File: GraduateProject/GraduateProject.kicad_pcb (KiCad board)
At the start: 2 copper layers, 90 x 80 mm, 143 parts, among them IC1 PIC16C620A-04/SS, IC2 PIC16C620A-04/SS, J1 Conn_01x05_Pin, J2 Conn_01x04_Pin, J5 Conn_01x04_Pin, J6 Conn_01x04_Pin, J7 Conn_01x05_Pin, J8 Conn_01x05_Pin, Q1 MMBT2222A, Q10 IMX1T110, Q11 MMBT2222A, Q12 IMX1T110, Q13 IMX1T110, Q14 IMX1T110, Q15 IMX1T110, Q16 MMBT2222A, Q17 MMBT2222A, Q18 MMBT2222A, Q19 MMBT2222A, Q2 MMBT2222A, Q20 MMBT2222A, Q21 MMBT2222A, Q22 MMBT2222A, Q23 MMBT3906, Q24 MMBT2222A, Q25 MMBT2222A, Q26 MMBT3906, Q27 MMBT2222A, Q28 MMBT2222A, Q29 MMBT2222A, Q3 MBT3946DW1T1, Q30 MMBT2222A, Q31 MMBT2222A, Q32 MMBT2222A, Q33 MMBT2222A, Q34 MMBT2222A, Q35 MMBT2222A, Q36 MMBT2222A, Q4 MMBT2222A, Q6 IMX1T110, Q7 IMX1T110, Q8 MBT3946DW1T1, Q9 IMX1T110, SW1 SS12D10G3, U2 L7815, U3 L7805, U4 L7805, U5 B0505S-1W, U6 EL357N(D)(TA)-G_C42385002, U7 B0505S-1W

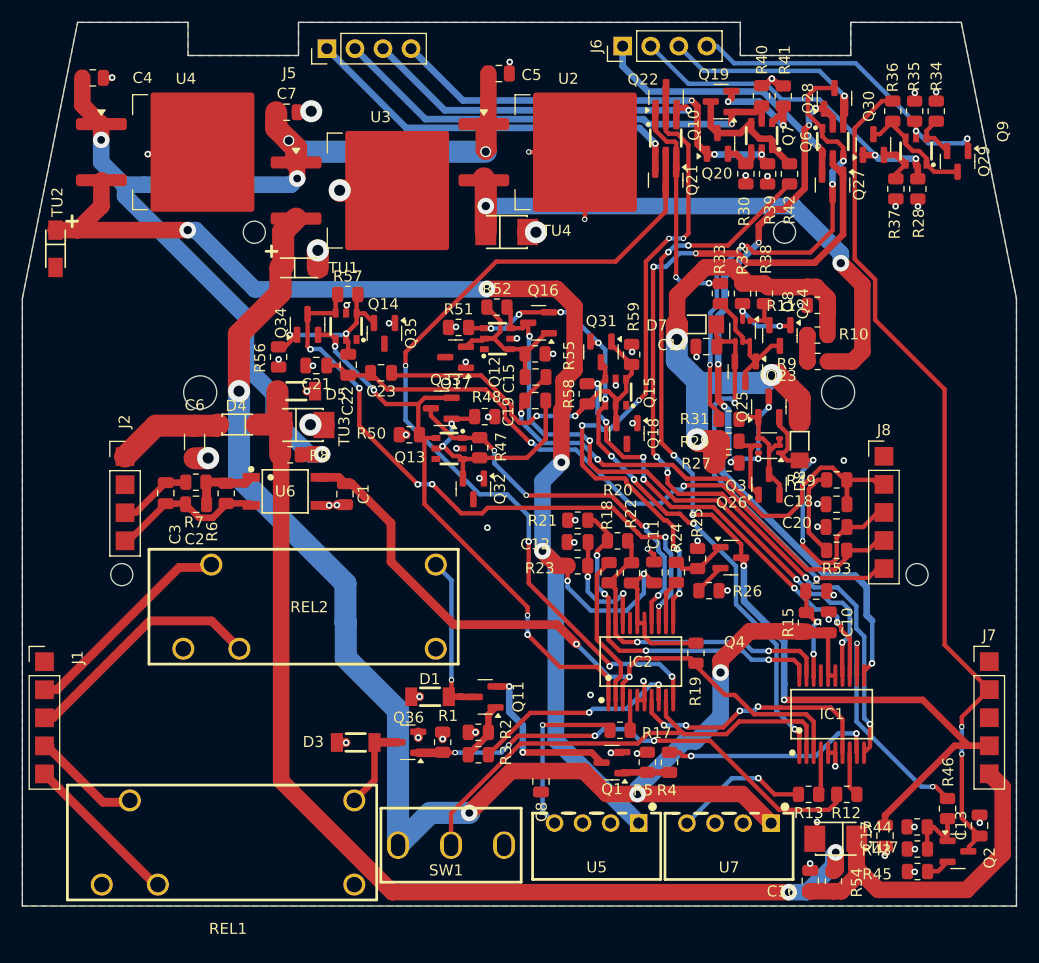
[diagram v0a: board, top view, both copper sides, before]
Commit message: Add files via upload
5/10/25
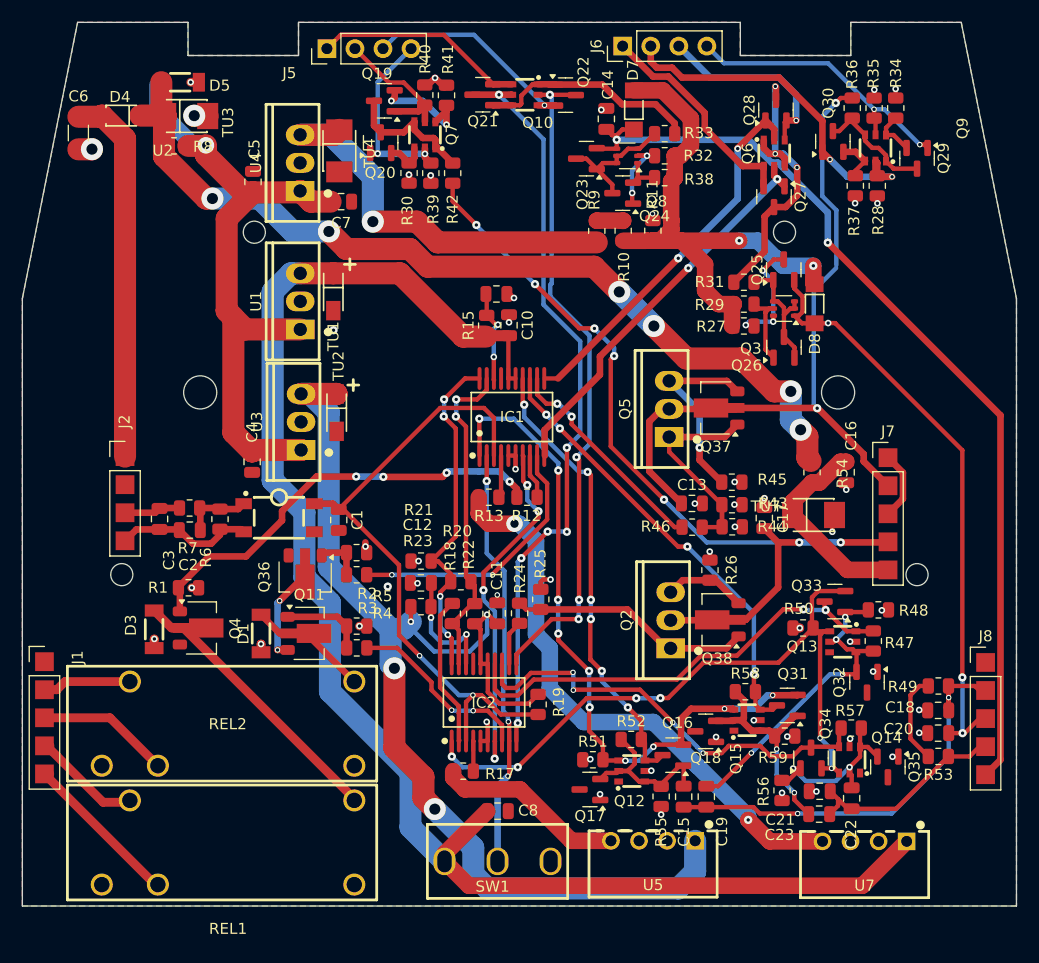
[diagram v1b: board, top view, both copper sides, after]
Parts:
- removed Q1: MMBT2222A, Package_TO_SOT_SMD:SOT-23
- removed U6: EL357N(D)(TA)-G_C42385002, easyeda2kicad:SOP-4_L3.9-W4.4-P2.54-LS7.0-TL
- added Q37: BCX56, Package_TO_SOT_SMD:SOT-89-3, F.Cu at (167.8, 114.9)
- added Q38: BCX56, Package_TO_SOT_SMD:SOT-89-3, F.Cu at (167.9, 134.1)
- added Q5: TIP110G, easyeda2kicad:TO-220-3_L10.0-W4.5-P2.54-L, F.Cu at (163.6, 115.0)
- added U1: LM7805T, easyeda2kicad:TO-220-3_L10.0-W4.5-P2.54-L, F.Cu at (130.2, 105.3)
- Q11, Q36, Q4: value MMBT2222A -> BCX56; footprint Package_TO_SOT_SMD:SOT-23 -> Package_TO_SOT_SMD:SOT-89-3
- Q2: value MMBT2222A -> TIP110G; footprint Package_TO_SOT_SMD:SOT-23 -> easyeda2kicad:TO-220-3_L10.0-W4.5-P2.54-L
- U2: value L7815 -> TLP181GB-S; footprint Package_TO_SOT_SMD:TO-263-2 -> easyeda2kicad:SOP-4_L3.7-W4.6-P2.54-LS7.0-TL
- U3: value L7805 -> LM7805T; footprint Package_TO_SOT_SMD:TO-263-2 -> easyeda2kicad:TO-220-3_L10.0-W4.5-P2.54-L
- U4: value L7805 -> L7815CV; footprint Package_TO_SOT_SMD:TO-263-2 -> easyeda2kicad:TO-220-3_L10.0-W4.5-P2.54-L
- moved C22 60.1 mm to (180.1, 150.2)
- moved Q34 60.1 mm to (176.4, 146.6)
- moved R56 60.1 mm to (173.8, 149.5)
- moved Q14 60.1 mm to (179.9, 146.8)
- moved R57 60.1 mm to (180.0, 143.9)
- moved Q35 60.1 mm to (183.4, 147.4)
- moved C21 59.7 mm to (177.2, 149.6)
- moved C23 56.3 mm to (177.1, 151.7), turned to 0 degrees
- moved Q4 48.3 mm to (121.2, 134.8)
- moved U2 42.2 mm to (128.2, 124.8)
- moved R55 41.7 mm to (162.8, 150.1), turned to -90 degrees
- moved Q16 41.0 mm to (163.9, 146.3)
- moved R52 41.0 mm to (160.1, 144.9)
- moved Q12 41.0 mm to (160.2, 147.8)
- moved Q17 41.0 mm to (156.4, 149.4)
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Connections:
- C13 pad 1: Net-(J7-Pin_2) -> /CONNECTORS/BCX56_2
- C2 pad 2: Net-(U6-AN) -> Net-(U2-AN)
- C4 pad 1: Net-(U2-IN) -> Net-(U1-VIN)
- C5 pad 1: Net-(U2-IN) -> Net-(U1-VIN)
- C7 pad 1: Net-(U2-IN) -> Net-(U1-VIN)
- J7 pad 1: unconnected-(J7-Pin_1-Pad1) -> Net-(J7-Pin_1)
- J7 pad 2: Net-(J7-Pin_2) -> /CONNECTORS/BCX56_2
- J7 pad 3: unconnected-(J7-Pin_3-Pad3) -> Net-(J7-Pin_1)
- Q11 pad 2: Net-(Q1-C) -> Net-(D1-C)
- Q11 pad 3: Net-(D1-C) -> Net-(Q11-E)
- Q2 pad 1: Net-(Q2-B) -> /PICs/BCX56_38_1
- Q2 pad 2: Net-(Q2-E) -> /CONNECTORS/CONN_J3_4
- Q2 pad 3: Net-(J7-Pin_2) -> /PICs/BCX56_38_3
- Q36 pad 1: /PICs/RB1_PIC1 -> Net-(Q36-B)
- Q36 pad 2: GND -> Net-(Q11-E)
- Q36 pad 3: Net-(D3-C) -> GND
- Q4 pad 1: Net-(Q4-B) -> /PICs/RB1_PIC1
- Q4 pad 2: Net-(Q4-E) -> Net-(D3-C)
- Q4 pad 3: /CONNECTORS/CONN_J3_4 -> GND
- R24 pad 1: Net-(Q4-B) -> /PICs/BCX56_38_1
- R25 pad 1: Net-(Q4-B) -> /PICs/BCX56_38_1
- R26 pad 1: Net-(Q4-E) -> /PICs/BCX56_38_3
- R36 pad 2: Net-(J7-Pin_2) -> /CONNECTORS/BCX56_2
- R4 pad 2: Net-(Q1-B) -> Net-(Q36-B)
- R43 pad 1: Net-(Q2-B) -> /CONNECTORS/BCX56_1
- R44 pad 1: Net-(Q2-B) -> /CONNECTORS/BCX56_1
- R45 pad 1: Net-(Q2-E) -> /CONNECTORS/BCX56_3
- R46 pad 1: Net-(Q2-B) -> /CONNECTORS/BCX56_1
- R5 pad 2: Net-(Q1-B) -> Net-(Q36-B)
- R6 pad 1: Net-(U6-AN) -> Net-(U2-AN)
- R7 pad 2: Net-(U6-AN) -> Net-(U2-AN)
- R8 pad 1: Net-(U2-IN) -> Net-(U1-VIN)
- R9 pad 1: Net-(U2-OUT) -> Net-(U4-OUT)
- TU4 pad 1: Net-(U2-OUT) -> Net-(U4-OUT)
- U2 pad 1: Net-(U2-IN) -> Net-(U2-AN)
- U2 pad 3: Net-(U2-OUT) -> Net-(J2-Pin_4)
- U3 pad 1: Net-(U2-IN) -> Net-(U1-VIN)
- U3 pad 3: /PICs/5V_PIC1 -> /PICs/5V_PIC2
- U4 pad 1: Net-(U2-IN) -> Net-(U1-VIN)
- U4 pad 3: /PICs/5V_PIC2 -> Net-(U4-OUT)
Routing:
- net Net-(U2-IN): track 98.9 -> 0.00 mm, vias 5 -> 0
- net Net-(J7-Pin_2): track 77.2 -> 0.00 mm, vias 2 -> 0
- net /CONNECTORS/BCX56_2: track 0.00 -> 65.7 mm, vias 0 -> 2
- net Net-(U1-VIN): track 0.00 -> 64.5 mm, vias 0 -> 1
- net Net-(U2-OUT): track 52.1 -> 0.00 mm, vias 2 -> 0
- net /CONNECTORS/CONN_J2_5: track 37.0 -> 85.7 mm
- net /CONNECTORS/RB3_PIC1: track 82.6 -> 36.0 mm, vias 6 -> 2
- net /CONNECTORS/CONN_J2_4: track 61.1 -> 18.2 mm, vias 2 -> 0
- net Net-(U7-Vo): track 12.4 -> 52.2 mm, vias 1 -> 2
- net Net-(U4-OUT): track 0.00 -> 37.0 mm, vias 0 -> 1
- net /CONNECTORS/RB4_PIC1: track 67.1 -> 35.2 mm, vias 6 -> 2
- net GND: track 72.8 -> 42.8 mm, vias 66 -> 52
- net /CONNECTORS/Q7_B1: track 42.5 -> 13.0 mm, vias 1 -> 0
- net /PICs/5V_PIC2: track 135.5 -> 107.4 mm, vias 6 -> 4
- net /CONNECTORS/CONN_J2_3: track 26.0 -> 53.3 mm, vias 2 -> 3
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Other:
- board text added: "30mm"
- board text added: "55mm"
- board text added: "61mm"
- board text removed: "70mm"
